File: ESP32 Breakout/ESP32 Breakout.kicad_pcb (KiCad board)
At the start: 2 copper layers, 49 x 22 mm, 9 parts, among them J1 Conn_01x05_Socket, J2 Conn_01x02_Socket, Q1 2N3904, U1 ESP32C3

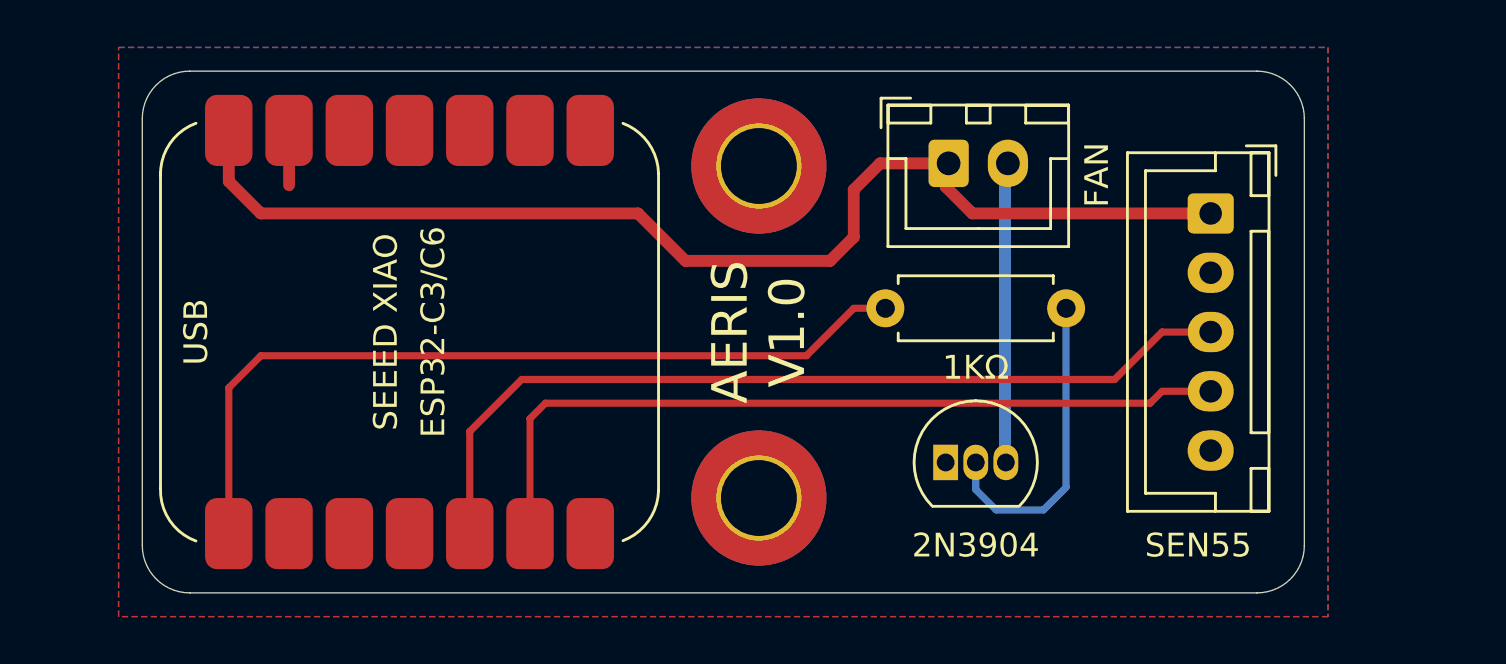
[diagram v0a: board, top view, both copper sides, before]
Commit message: Update to V1.1
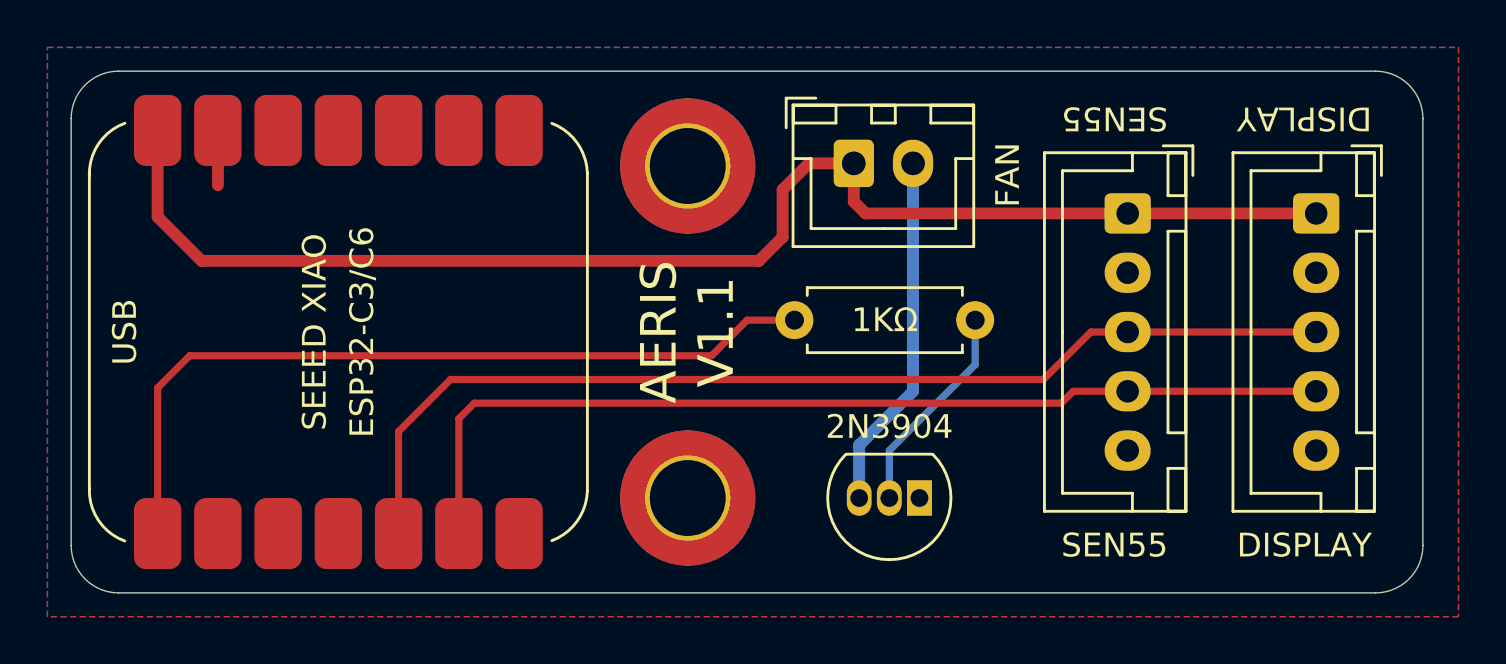
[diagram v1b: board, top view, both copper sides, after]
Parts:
- added J3: Conn_01x05_Socket, Custom Footprints:JST_XH_B5B-XH-A_1x05_P2.50mm_Vertical, F.Cu at (173.5, 95.0)
- moved J2 4.00 mm to (154.0, 92.9)
- moved R1 3.87 mm to (151.5, 99.5)
- moved J1 3.50 mm to (165.6, 95.0)
- moved REF** 3.00 mm to (125.9, 100.0)
- moved REF** 3.00 mm to (147.0, 93.0)
- moved REF** 3.00 mm to (147.0, 107.0)
- moved REF** 3.00 mm to (134.9, 100.0)
- moved U1 3.00 mm to (132.3, 100.0)
- moved Q1 1.86 mm to (156.8, 107.0), turned to 180 degrees
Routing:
- net /SCL: track 6.48 -> 16.7 mm
- net +5V: track 49.3 -> 58.0 mm
- net /SDA: track 37.3 -> 44.7 mm
- net Net-(Q1-B): track 12.7 -> 8.50 mm
- net Net-(J2-Pin_2): track 12.8 -> 14.6 mm
- net /PWM: track 35.2 -> 34.2 mm
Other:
- board size 49 x 22 mm -> 57 x 22 mm
- board text added: "AERIS V1.1"
- board text added: "DISPLAY"
- board text added: "M3x4 BHCS"
- board text removed: "AERIS V1.0"
- board text removed: "M3x6 BHCS"
